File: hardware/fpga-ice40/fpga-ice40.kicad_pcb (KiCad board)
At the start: 4 copper layers, 53.3 x 48.6 mm, 88 parts, among them J1 Conn_01x03, J2 MicroSD_Molex_1040310811, J3 FTSH-105-01-L-DV-K, J4 FTSH-105-01-L-DV-K, J5 USB_B_Micro, J6 Conn_02x20_Odd_Even, Q1 2N7002H-7, U1 iCE40HX4K-TQ144, U10 MC74HC1G08DTT1G, U2 AZ1117-3.3, U3 AZ1117-1.2, U4 IS42S16320F-7TL, U5 S25FL256SAGMFI01, U6 W25Q32JVSS, U7 S25FL256SAGMFI01, U8 W25Q32JVSS, U9 FT245RL, X1 50MHz

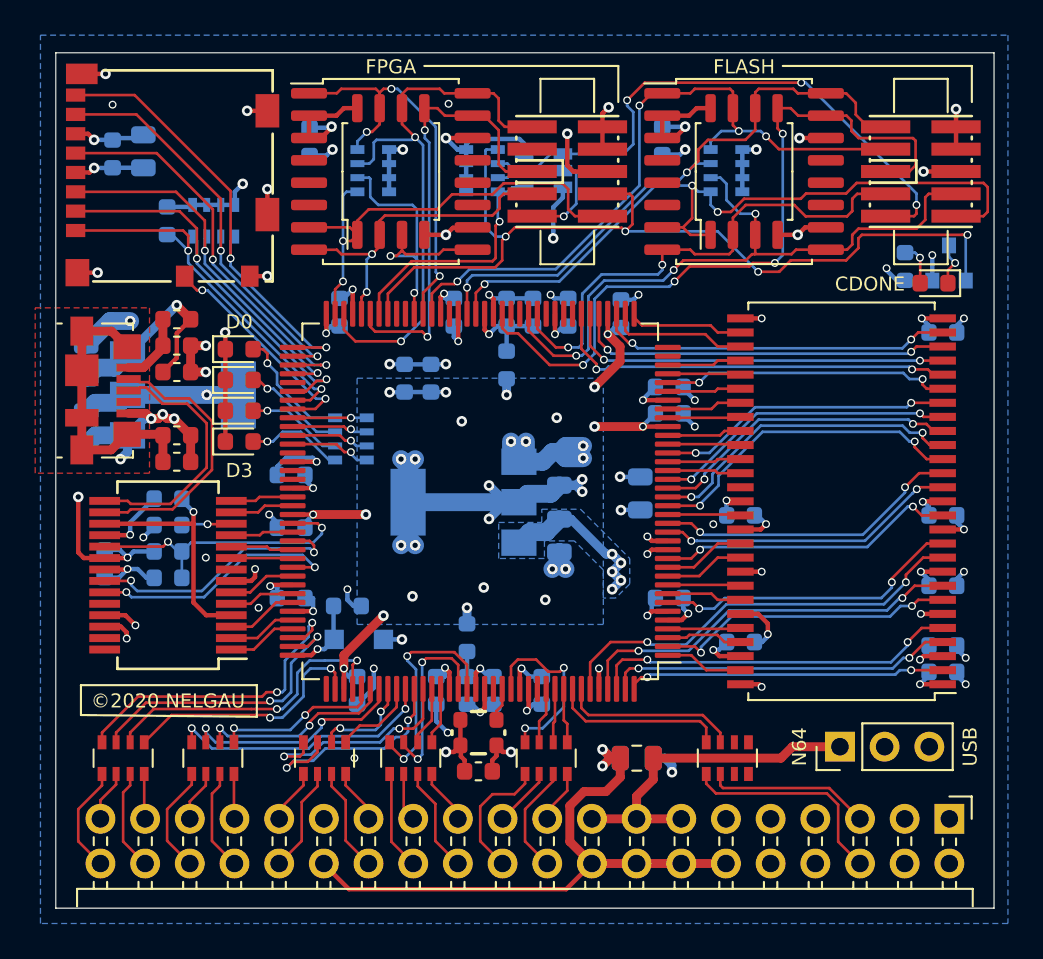
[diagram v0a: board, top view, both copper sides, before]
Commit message: Completed verification of all pins for all symbols
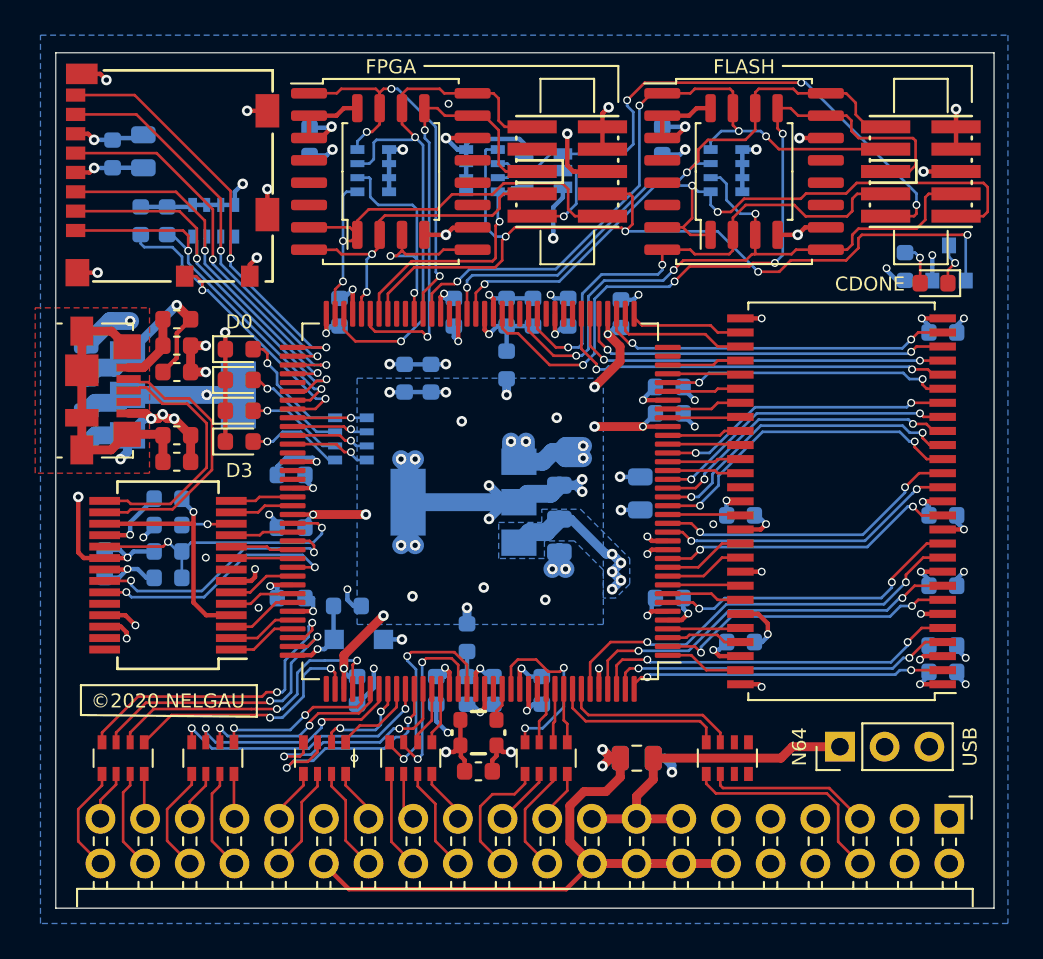
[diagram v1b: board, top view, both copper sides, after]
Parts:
- added R8: 10k, Resistor_SMD:R_0603_1608Metric, B.Cu at (140.7, 79.0)
- U5, U7: value S25FL256SAGMFI01 -> S25FL256SAGMFI01x
- U6, U8: value W25Q32JVSS -> W25Q32JVSSIM
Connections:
- net SD_CD renamed SD_DET
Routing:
- net SD_DET: track 13.1 -> 18.8 mm
- net P3V3: track 103.7 -> 105.2 mm
- net GND: track 168.1 -> 168.5 mm, vias 73 -> 72
